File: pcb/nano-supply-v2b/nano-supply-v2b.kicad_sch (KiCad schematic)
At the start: 49 parts, among them J1 USB_C_Receptacle_USB2.0_16P, J2 Conn_01x03_Pin, J3 IDC 2x8 SMD, J4 IDC 2x8 SMD, J5 IDC 2x8 SMD, J6 IDC 2x8 SMD, J7 IDC 2x8 SMD, J8 IDC 2x8 SMD, J9 Conn_01x02_Pin, Q1 AONR21307, U1 HUSB238_xxxDD

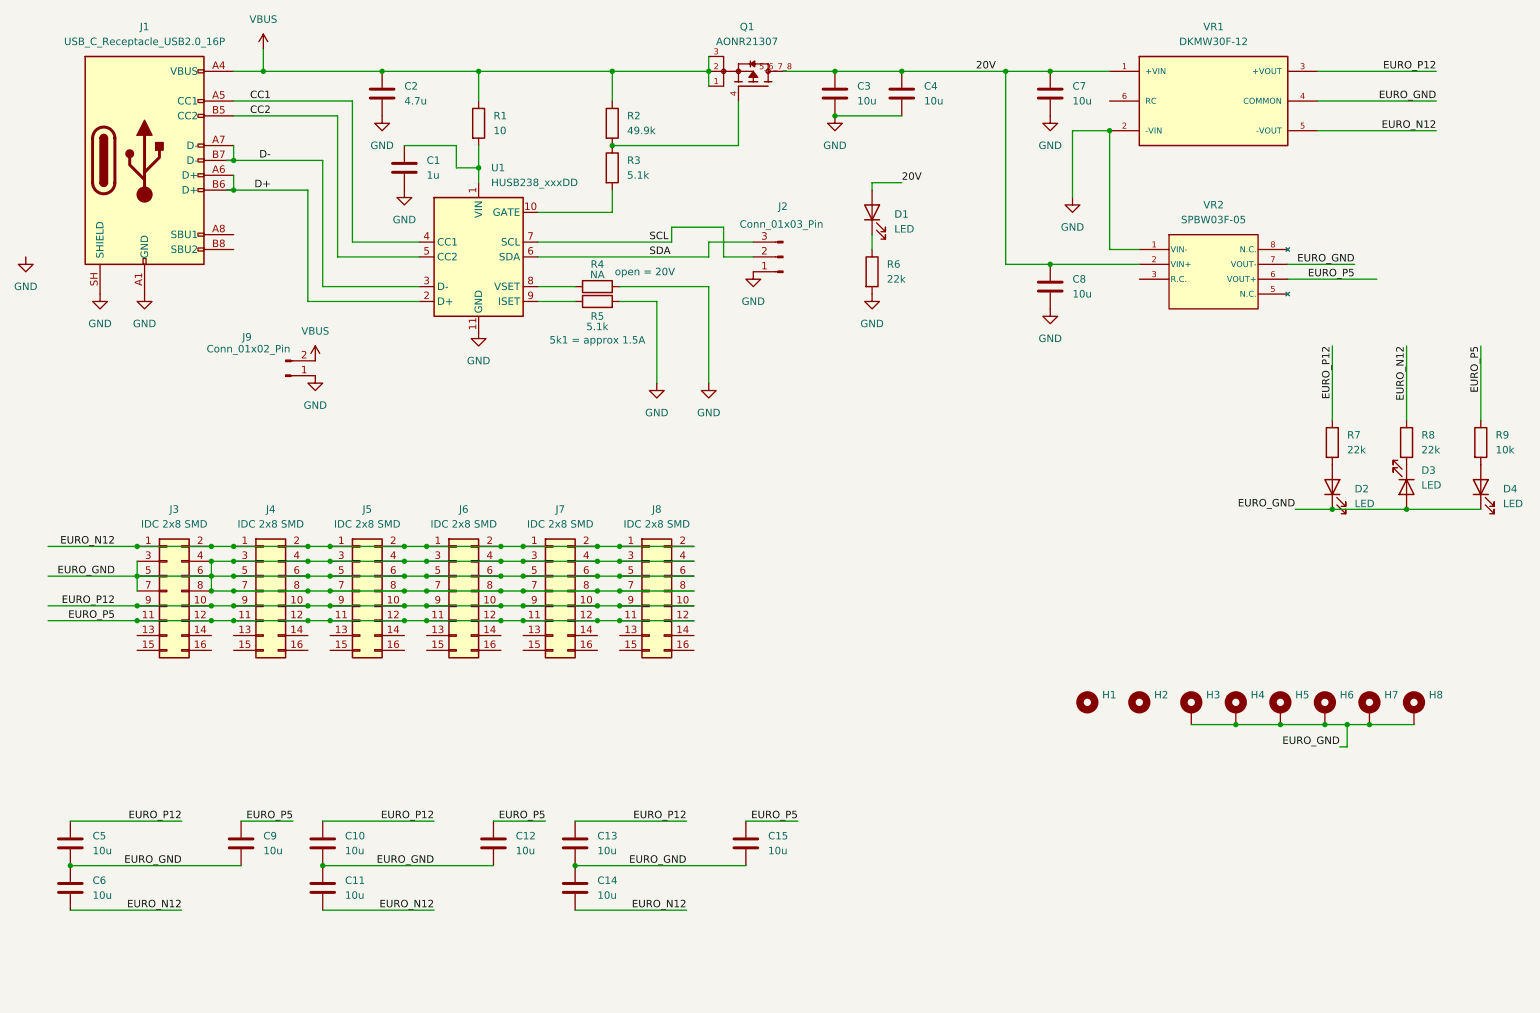
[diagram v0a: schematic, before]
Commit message: basic board routing
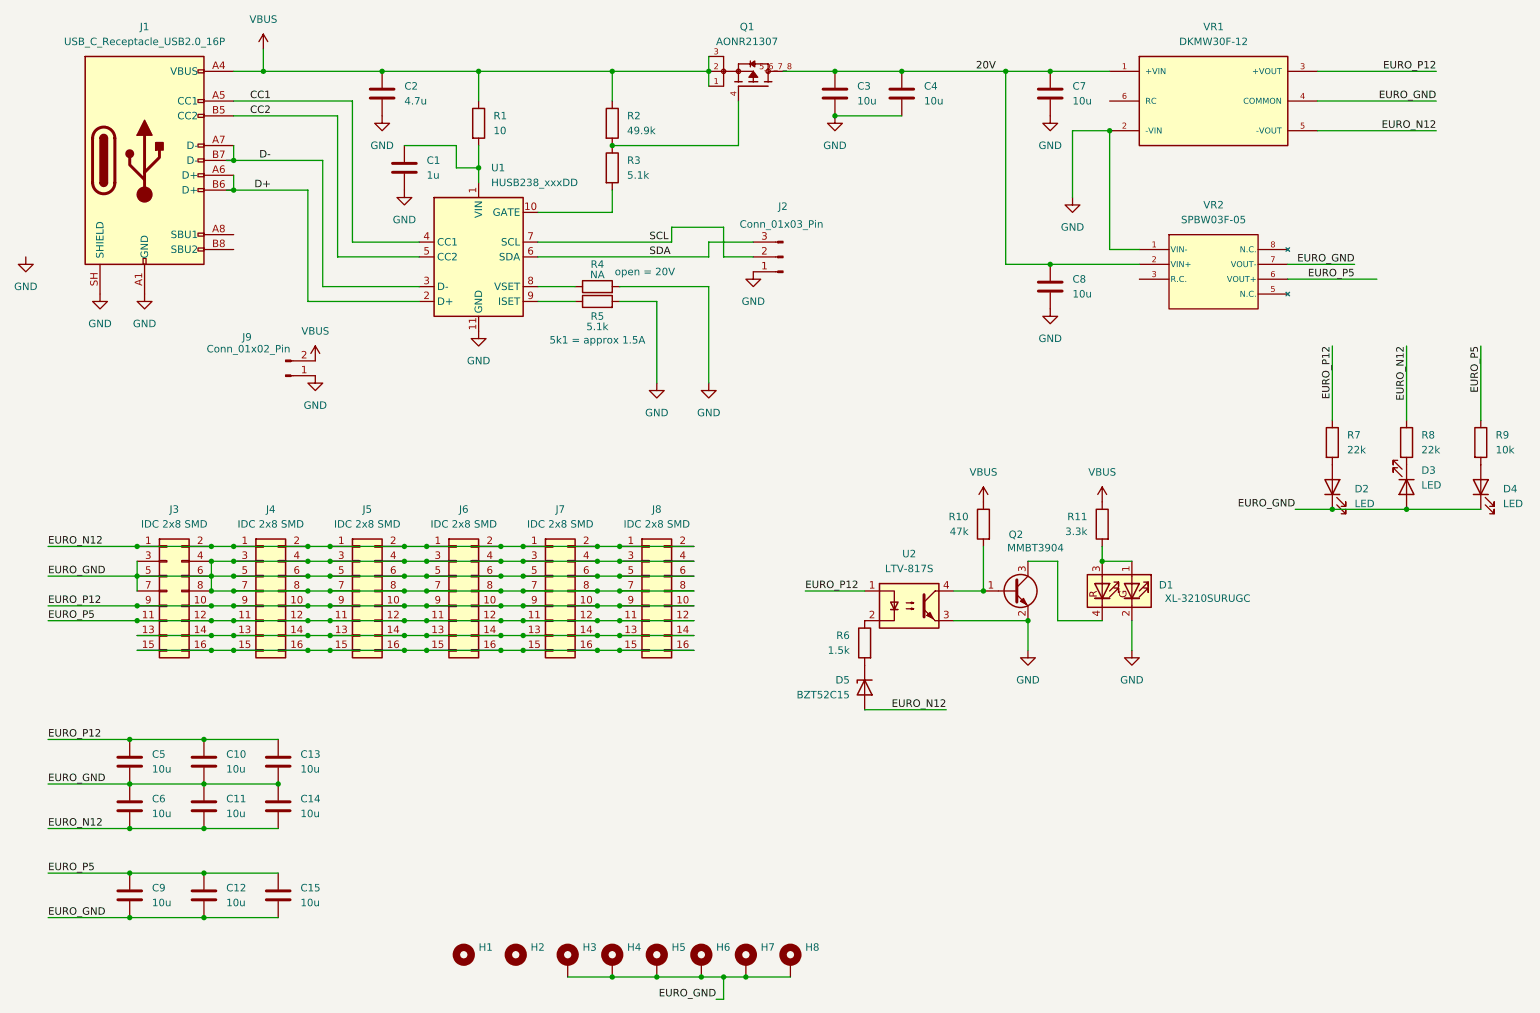
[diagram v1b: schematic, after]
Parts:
- removed D1: LED, LED_SMD:LED_Kingbright_APA1606_1.6x0.6mm_Horizontal, symbol Device:LED
- added D1: XL-3210SURUGC, nano-supply:XL-3210SURUGC, symbol nano-supply:XL-3210SURUGC
- added D5: BZT52C15, Diode_SMD:D_SOD-123, symbol Device:D_Zener
- added Q2: MMBT3904, Package_TO_SOT_SMD:SOT-23, symbol Transistor_BJT:MMBT3904
- added R10: 47k, Resistor_SMD:R_0603_1608Metric, symbol Device:R
- added R11: 3.3k, Resistor_SMD:R_0805_2012Metric, symbol Device:R
- added U2: LTV-817S, Package_DIP:SMDIP-4_W9.53mm, symbol Isolator:LTV-817S
- R6: value 22k -> 1.5k; footprint Resistor_SMD:R_0603_1608Metric -> Resistor_SMD:R_0805_2012Metric; LCSC C31850 -> C23186
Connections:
- net EURO_N12: now also D5.2 (A)
- net EURO_P12: now also U2.1
- net GND: now also D1.2 (GK), Q2.2 (E), U2.3; no longer R6.2
- net VBUS: now also R10.1, R11.1
- net at J7.13 (Pin_13): now also J3.13 (Pin_13), J3.14 (Pin_14), J4.13 (Pin_13), J4.14 (Pin_14), J5.13 (Pin_13), J5.14 (Pin_14), J6.13 (Pin_13), J6.14 (Pin_14), J7.14 (Pin_14), J8.13 (Pin_13), J8.14 (Pin_14)
- net at J7.15 (Pin_15): now also J3.15 (Pin_15), J3.16 (Pin_16), J4.15 (Pin_15), J4.16 (Pin_16), J5.15 (Pin_15), J5.16 (Pin_16), J6.15 (Pin_15), J6.16 (Pin_16), J7.16 (Pin_16), J8.15 (Pin_15), J8.16 (Pin_16)
- net at R6.1: now also U2.2
- new net: D1.1 (GA), D1.3 (RA), R11.2
- new net: D1.4 (RK), Q2.3 (C)
- new net: D5.1 (K), R6.2
- new net: Q2.1 (B), R10.2, U2.4
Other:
- moved on the sheet: C10, C11, C12, C13, C14, C15, C5, C6, C9, H1, H2, H3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
